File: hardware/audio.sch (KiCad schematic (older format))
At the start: 25 parts, among them U4 FM8002A, U5 TM8211, U6 FM8002A

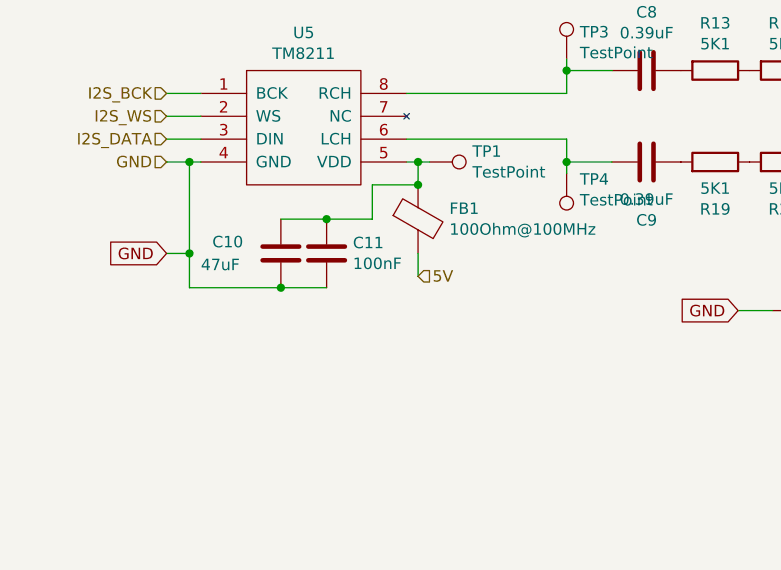
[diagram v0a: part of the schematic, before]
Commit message: Rev5 schematic changes and pcb cleanup
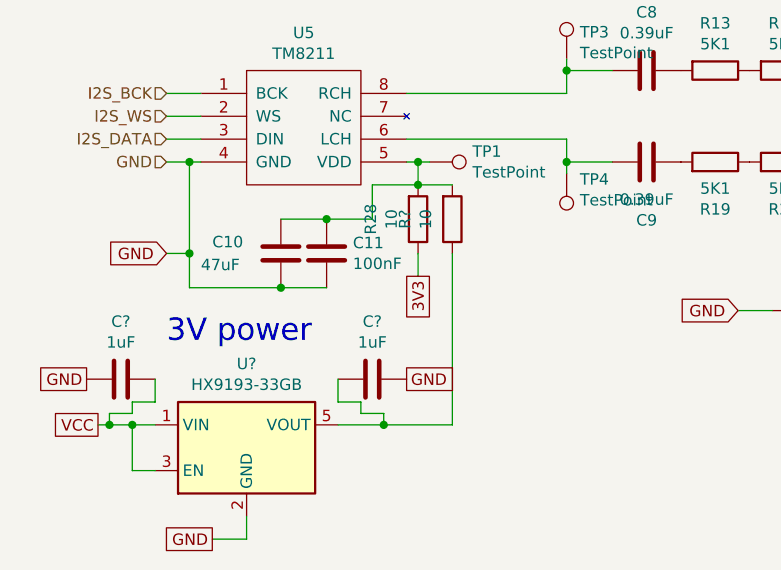
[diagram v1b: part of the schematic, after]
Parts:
- removed FB1: 100Ohm@100MHz, Inductor_SMD:L_0805_2012Metric, symbol Device:Ferrite_Bead
- added C? (x2): 1uF, Capacitor_SMD:C_0603_1608Metric, symbol Device:C
- added R28, R?: 10, Resistor_SMD:R_0603_1608Metric, symbol Device:R
- added U?: HX9193-33GB, Package_TO_SOT_SMD:SOT-23-5, symbol Regulator_Linear:MIC5504-3.3YM5
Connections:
- net GND: now also C?.1, C?.2, U?.2 (GND)
- net at C10.1, C11.1, TP1.1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: now also R28.2, R?.2
- new net: C?.1, R?.1, U?.5 (VOUT)
- new net 3V3: R28.1
- new net VCC: C?.2, U?.1 (VIN), U?.3 (EN)
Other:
- note added: "3V power"
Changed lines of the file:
@@
 	1300 3450 1400 3450
-Wire Wire Line
-	2400 3550 2400 3450
 Wire Wire Line
 	2400 3450 2350 3450
@@
 Wire Wire Line
 	2400 3950 2400 3850
-Text HLabel 2400 3950 2    50   Input ~ 0
-5V
 $Comp
 L Device:C C11
@@
 	1    0    0    -1
 $EndComp
-$Comp
-L Device:Ferrite_Bead FB1
-U 1 1 5DF0F498
-P 2400 3700
-F 0 "FB1" H 2537 3746 50  0000 L CNN
-F 1 "100Ohm@100MHz" H 2537 3655 50  0000 L CNN
-F 2 "Inductor_SMD:L_0805_2012Metric" V 2330 3700 50  0001 C CNN
-F 3 "~" H 2400 3700 50  0001 C CNN
-F 4 "C1017" H 2400 3700 50  0001 C CNN "LCSC"
-	1    2400 3700
-	1    0    0    -1
-$EndComp
 Wire Wire Line
 	6150 2300 6500 2300
@@
 Wire Wire Line
 	2400 3550 2200 3550
-Connection ~ 2400 3550
 Text HLabel 7050 3900 1    50   Input ~ 0
 5V
@@
 	3050 3500 3050 3450
 Connection ~ 3050 3450
+Text GLabel 2400 3950 3    50   UnSpc ~ 0
+3V3
+$Comp
+L Device:R R28
+U 1 1 5EE31536
+P 2400 3700
+F 0 "R28" V 2193 3700 50  0000 C CNN
+F 1 "10" V 2284 3700 50  0000 C CNN
+F 2 "Resistor_SMD:R_0603_1608Metric" V 2330 3700 50  0001 C CNN
+F 3 "~" H 2400 3700 50  0001 C CNN
+F 4 "" H 2400 3700 50  0001 C CNN "LCSC"
+	1    2400 3700
+	1    0    0    1
+$EndComp
+Connection ~ 2400 3550
+Wire Wire Line
+	2400 3450 2400 3550
+Text GLabel 1000 4600 0    50   UnSpc ~ 0
+VCC
+Wire Wire Line
+	1000 4600 1050 4600
+Text GLabel 1500 5100 0    50   UnSpc ~ 0
+GND
+Text Notes 1300 4250 0    98   ~ 0
+3V power
+$Comp
+L Device:C C?
+U 1 1 5EE458A4
+P 1100 4400
+AR Path="/5EE458A4" Ref="C?"  Part="1"
+AR Path="/5E4377A8/5EE458A4" Ref="C?"  Part="1"
+AR Path="/5E464BBE/5EE458A4" Ref="C?"  Part="1"
+F 0 "C?" V 848 4400 50  0000 C CNN
+F 1 "1uF" V 939 4400 50  0000 C CNN
+F 2 "Capacitor_SMD:C_0603_1608Metric" H 1138 4250 50  0001 C CNN
+F 3 "~" H 1100 4400 50  0001 C CNN
+F 4 "C15849" H 1100 4400 50  0001 C CNN "LCSC"
+	1    1100 4400
+	0    -1   1    0
+$EndComp
+$Comp
+L Device:C C?
+U 1 1 5EE458AB
+P 2200 4400
+AR Path="/5EE458AB" Ref="C?"  Part="1"
+AR Path="/5E4377A8/5EE458AB" Ref="C?"  Part="1"
+AR Path="/5E464BBE/5EE458AB" Ref="C?"  Part="1"
+F 0 "C?" V 1948 4400 50  0000 C CNN
+F 1 "1uF" V 2039 4400 50  0000 C CNN
+F 2 "Capacitor_SMD:C_0603_1608Metric" H 2238 4250 50  0001 C CNN
+F 3 "~" H 2200 4400 50  0001 C CNN
+F 4 "C15849" H 2200 4400 50  0001 C CNN "LCSC"
+	1    2200 4400
+	0    -1   1    0
+$EndComp
+Text GLabel 950  4400 0    50   UnSpc ~ 0
+GND
+Wire Wire Line
+	1250 4400 1250 4500
+Wire Wire Line
+	1250 4500 1150 4500
+Wire Wire Line
+	1150 4500 1150 4550
+Wire Wire Line
+	1150 4550 1050 4550
+Wire Wire Line
+	1050 4550 1050 4600
+Connection ~ 1050 4600
+Wire Wire Line
+	2050 4400 2050 4500
+Wire Wire Line
+	2050 4500 2150 4500
+Wire Wire Line
+	2150 4500 2150 4550
+Wire Wire Line
+	2150 4550 2250 4550
+Wire Wire Line
+	2250 4550 2250 4600
+Connection ~ 2250 4600
+Text GLabel 2350 4400 2    50   UnSpc ~ 0
+GND
+$Comp
+L Regulator_Linear:MIC5504-3.3YM5 U?
+U 1 1 5EE458C0
+P 1650 4700
+F 0 "U?" H 1650 5067 50  0000 C CNN
+F 1 " HX9193-33GB" H 1650 4976 50  0000 C CNN
+F 2 "Package_TO_SOT_SMD:SOT-23-5" H 1650 4300 50  0001 C CNN
+F 3 "" H 1400 4950 50  0001 C CNN
+F 4 "C296123" H 1650 4700 50  0001 C CNN "LCSC"
+	1    1650 4700
+	1    0    0    -1
+$EndComp
+Wire Wire Line
+	2050 4600 2250 4600
+Wire Wire Line
+	1050 4600 1150 4600
+Wire Wire Line
+	1650 5100 1650 5000
+Wire Wire Line
+	1500 5100 1650 5100
+Wire Wire Line
+	1250 4800 1150 4800
+Wire Wire Line
+	1150 4800 1150 4600
+Connection ~ 1150 4600
+Wire Wire Line
+	1150 4600 1250 4600
+$Comp
+L Device:R R?
+U 1 1 5EE48409
+P 2550 3700
+F 0 "R?" V 2343 3700 50  0000 C CNN
+F 1 "10" V 2434 3700 50  0000 C CNN
+F 2 "Resistor_SMD:R_0603_1608Metric" V 2480 3700 50  0001 C CNN
+F 3 "~" H 2550 3700 50  0001 C CNN
+F 4 "" H 2550 3700 50  0001 C CNN "LCSC"
+	1    2550 3700
+	1    0    0    1
+$EndComp
+Wire Wire Line
+	2400 3550 2550 3550
+Wire Wire Line
+	2550 3850 2550 4600
+Wire Wire Line
+	2250 4600 2550 4600
 $EndSCHEMATC
